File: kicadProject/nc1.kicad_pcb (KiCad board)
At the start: 2 copper layers, 72 parts, among them J1 Conn_01x02, J2 Conn_01x03, J3 Conn_01x06_Female, Q1 AOB414, Q2 AOB414, Q4 BD911, U1 NCP1034, U2 NE5534, U3 NE5534

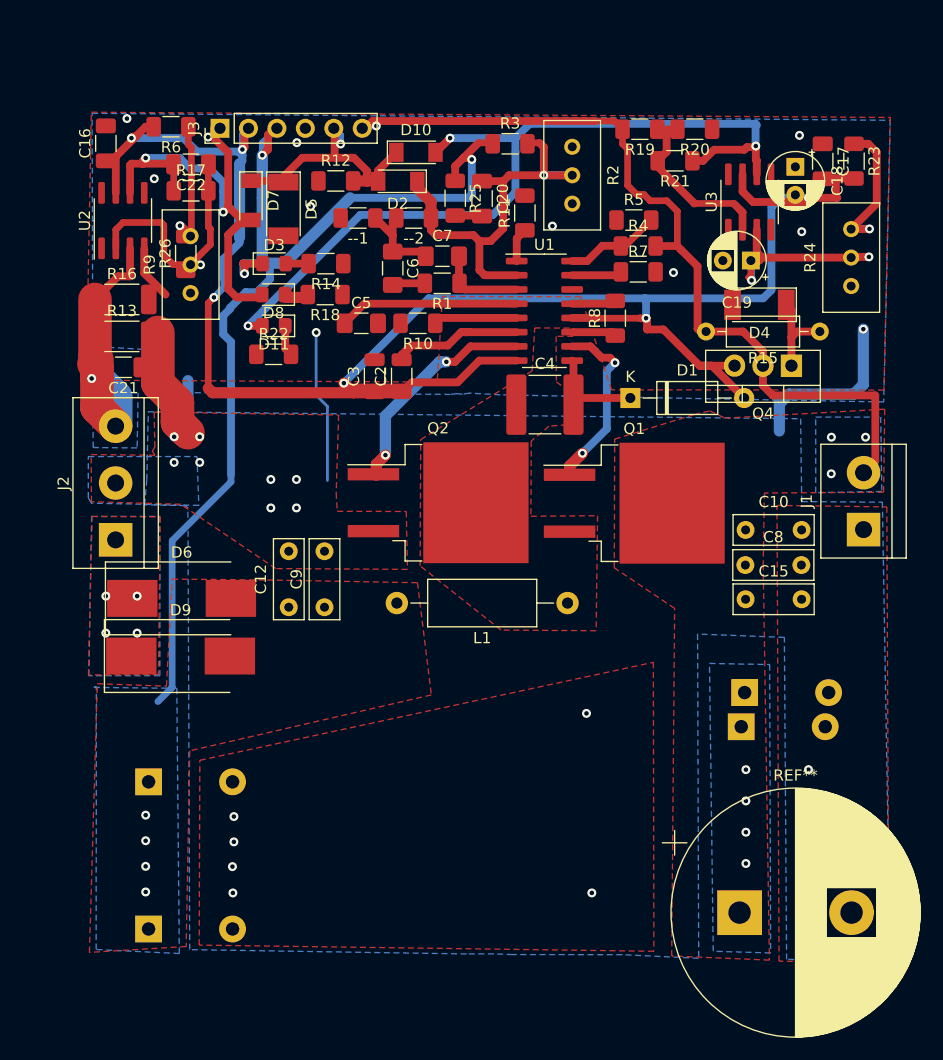
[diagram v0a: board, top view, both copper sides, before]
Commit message: V3
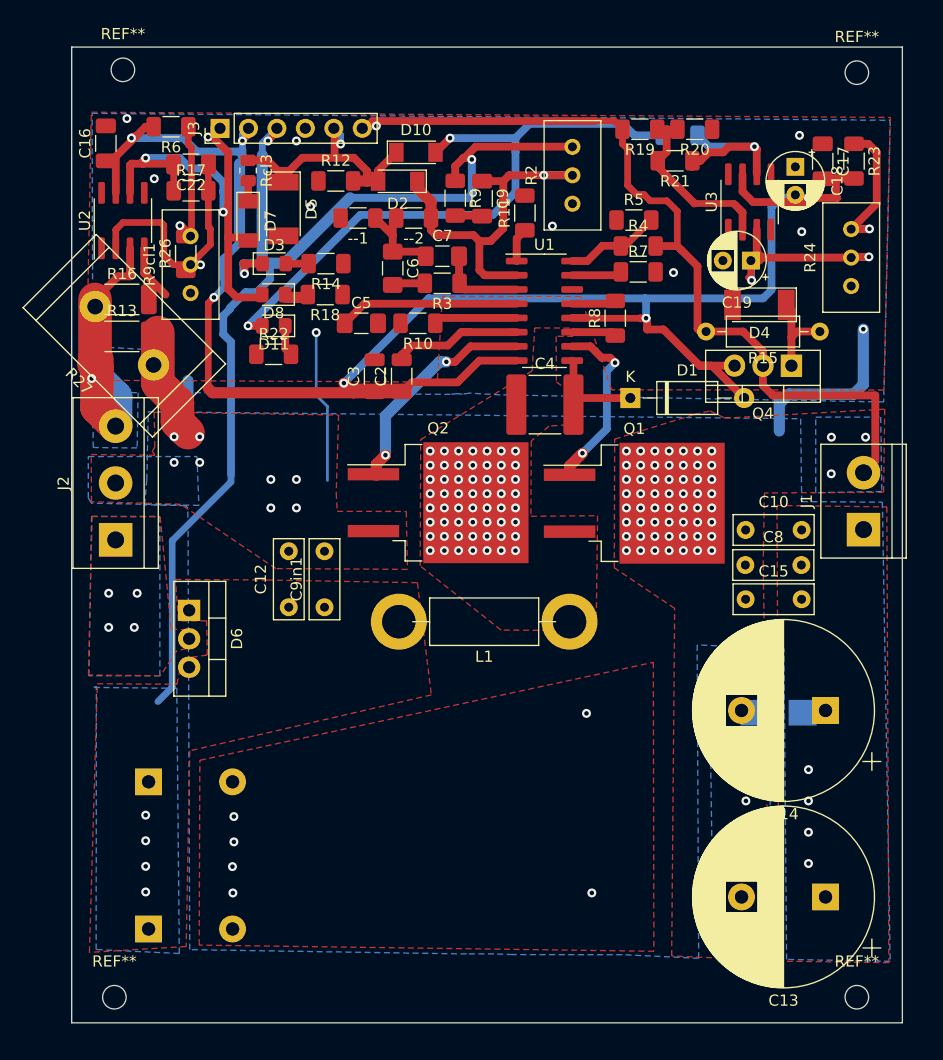
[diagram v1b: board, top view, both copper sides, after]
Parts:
- removed C21: 470n, Capacitor_SMD:C_1206_3216Metric_Pad1.33x1.80mm_HandSolder
- removed D9: 100v, Diode_SMD:D_SMC_Handsoldering
- removed the R3 at (56.2, 41.4)
- removed the REF** at (76.7, 110.0)
- added D12: SMBJ100A, Diode_SMD:D_SMB, B.Cu at (80.1, 92.2)
- added R27: 0.2 5W, Resistor_THT:R_Radial_Power_L16.1mm_W9.0mm_P7.37mm, F.Cu at (24.3, 61.1)
- added R28: 1k, Resistor_SMD:R_1206_3216Metric_Pad1.30x1.75mm_HandSolder, B.Cu at (71.3, 40.6)
- added REF**: MountingHole_2.1mm, MountingHole:MountingHole_2.1mm, F.Cu at (21.6, 34.8)
- added REF**: MountingHole_2.1mm, MountingHole:MountingHole_2.1mm, F.Cu at (87.1, 117.6)
- added REF**: MountingHole_2.1mm, MountingHole:MountingHole_2.1mm, F.Cu at (20.8, 117.6)
- added REF**: MountingHole_2.1mm, MountingHole:MountingHole_2.1mm, F.Cu at (87.1, 35.1)
- added Rcl3: 1k, Resistor_SMD:R_0805_2012Metric, F.Cu at (32.8, 43.8)
- --1: value R -> inf
- --2: value R -> 0
- C13: value 100n -> 10u; footprint Capacitor_THT:CP_Radial_D18.0mm_P7.50mm -> Capacitor_THT:CP_Radial_D16.0mm_P7.50mm; moved to F.Cu
- C14: value 100n -> 10u; moved to F.Cu
- C9: renamed from C20; value C -> 1094pF
- D6: value 100v -> Dout; footprint Diode_SMD:D_SMC_Handsoldering -> Package_TO_SOT_THT:TO-220-3_Vertical
- L1: value 100uH -> 45uH
- R11: value 4.7k -> 3.3k
- R2: value 20k -> 50k
- R3: renamed from R1; value R -> 150k
- R6: value 10k -> 18k
- R7: value 22k -> 18k
- R9: renamed from R25; value 47k -> 1.73k
- moved C13 17.0 mm to (84.3, 108.7), turned to 180 degrees
- moved C14 7.40 mm to (84.3, 92.0), turned to 180 degrees
- moved R2 5.08 mm to (61.7, 41.7), turned to 90 degrees
- moved D7 1.85 mm to (32.8, 48.3)
- moved L1 1.67 mm to (61.5, 84.1)
- moved D6 1.26 mm to (27.5, 83.1), turned to -90 degrees
- renumbered C9 to C9in1, R9 to R9cl1
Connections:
- C13 pad 1: Vin -> GND
- C13 pad 2: GND -> Vin
- C14 pad 1: Vin -> GND
- C14 pad 2: GND -> Vin
- D3 pad 2: Net-(D3-Pad2) -> GND
- D6 pad 1: Net-(D6-Pad1) -> Vout
- D6 pad 2: Vout -> Net-(J2-Pad1)
- D7 pad 1: FB -> Net-(D7-Pad1)
- J2 pad 1: Net-(D6-Pad1) -> Net-(J2-Pad1)
- R14 pad 1: GND -> Vout
- R14 pad 2: Net-(D3-Pad2) -> GND
- R2 pad 1: GND -> Vout
- R2 pad 3: Net-(R2-Pad3) -> GND
- R21 pad 1: Net-(D10-Pad2) -> Net-(R21-Pad1)
- U2 pad 1: Net-(U2-Pad1) -> unconnected-(U2-Pad1)
- U2 pad 8: Net-(U2-Pad8) -> unconnected-(U2-Pad8)
- U3 pad 1: Net-(U3-Pad1) -> unconnected-(U3-Pad1)
- U3 pad 6: Net-(D10-Pad2) -> Net-(R21-Pad1)
- U3 pad 8: Net-(U3-Pad8) -> unconnected-(U3-Pad8)
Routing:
- net Net-(D10-Pad2): track 75.5 -> 56.7 mm, vias 3 -> 2
- net Net-(R21-Pad1): track 0.00 -> 14.7 mm, vias 0 -> 1
- net Vout: track 95.9 -> 101.4 mm
- net Net-(--2-Pad1): track 36.9 -> 32.9 mm, vias 1 -> 2
- net Net-(D3-Pad2): track 2.05 -> 0.00 mm
- net GND: track 63.2 -> 65.1 mm, vias 29 -> 28
- net Net-(D7-Pad1): track 0.00 -> 1.83 mm
- net FB: track 22.9 -> 24.1 mm
- net Csense: track 40.5 -> 41.1 mm
- net 15V: track 176.0 -> 175.3 mm
- net Vin: vias 8 -> 64
- net Net-(J2-Pad1): vias 0 -> 4
- net Net-(D6-Pad1): vias 4 -> 0
- net Net-(C4-Pad1): vias 0 -> 56
- added copper zone on B.Cu, net Net-(C4-Pad1)
- added copper zone on B.Cu, net Net-(J2-Pad1)
- added copper zone on F.Cu, net Net-(J2-Pad1)
- removed copper zone on B.Cu, net Net-(D6-Pad1)
- removed copper zone on F.Cu, net Net-(D6-Pad1)
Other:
- board outline added: 74.2 x 87.1 mm
- net class Default removed
